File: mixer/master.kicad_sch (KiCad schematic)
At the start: 18 parts, among them J1 EURORACK_CONN_16, J2 AUX_OUT, J3 AUX_IN_R, J4 AUX_IN_L, J5 MAIN_OUT_R, J6 MAIN_OUT_L, U1 TL074

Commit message: making progress on the outline
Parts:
- C1, C2, C3, C4: footprint (none) -> Capacitor_SMD:C_0603_1608Metric
- R1, R2, R3, R4, R5: footprint (none) -> Resistor_SMD:R_0603_1608Metric
- U1: footprint (none) -> Package_SO:SOIC-14_3.9x8.7mm_P1.27mm
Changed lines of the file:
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@@
 			)
 		)
-		(property "Footprint" ""
+		(property "Footprint" "Resistor_SMD:R_0603_1608Metric"
 			(at 83.312 34.29 90)
 			(effects
@@
 			)
 		)
-		(property "Footprint" ""
+		(property "Footprint" "Capacitor_SMD:C_0603_1608Metric"
 			(at 275.2852 35.56 0)
 			(effects
@@
 			)
 		)
-		(property "Footprint" ""
+		(property "Footprint" "Resistor_SMD:R_0603_1608Metric"
 			(at 152.4 128.778 90)
 			(effects
@@
 			)
 		)
-		(property "Footprint" ""
+		(property "Footprint" "Package_SO:SOIC-14_3.9x8.7mm_P1.27mm"
 			(at 170.18 109.22 0)
 			(effects
@@
 			)
 		)
-		(property "Footprint" ""
+		(property "Footprint" "Capacitor_SMD:C_0603_1608Metric"
 			(at 33.9852 43.18 0)
 			(effects
@@
 			)
 		)
-		(property "Footprint" ""
+		(property "Footprint" "Resistor_SMD:R_0603_1608Metric"
 			(at 152.4 141.478 90)
 			(effects
@@
 			)
 		)
-		(property "Footprint" ""
+		(property "Footprint" "Resistor_SMD:R_0603_1608Metric"
 			(at 152.4 93.218 90)
 			(effects
@@
 			)
 		)
-		(property "Footprint" ""
+		(property "Footprint" "Capacitor_SMD:C_0603_1608Metric"
 			(at 20.0152 31.75 0)
 			(effects
@@
 			)
 		)
-		(property "Footprint" ""
+		(property "Footprint" "Package_SO:SOIC-14_3.9x8.7mm_P1.27mm"
 			(at 130.81 88.9 0)
 			(effects
@@
 			)
 		)
-		(property "Footprint" ""
+		(property "Footprint" "Package_SO:SOIC-14_3.9x8.7mm_P1.27mm"
 			(at 170.18 144.78 0)
 			(effects
@@
 			)
 		)
-		(property "Footprint" ""
+		(property "Footprint" "Resistor_SMD:R_0603_1608Metric"
 			(at 152.4 105.918 90)
 			(effects
@@
 			)
 		)
-		(property "Footprint" ""
+		(property "Footprint" "Package_SO:SOIC-14_3.9x8.7mm_P1.27mm"
 			(at 262.89 29.21 0)
 			(effects
@@
 			)
 		)
-		(property "Footprint" ""
+		(property "Footprint" "Package_SO:SOIC-14_3.9x8.7mm_P1.27mm"
 			(at 134.62 137.16 0)
 			(effects
@@
 			)
 		)
-		(property "Footprint" ""
+		(property "Footprint" "Capacitor_SMD:C_0603_1608Metric"
 			(at 33.9852 31.75 0)
 			(effects

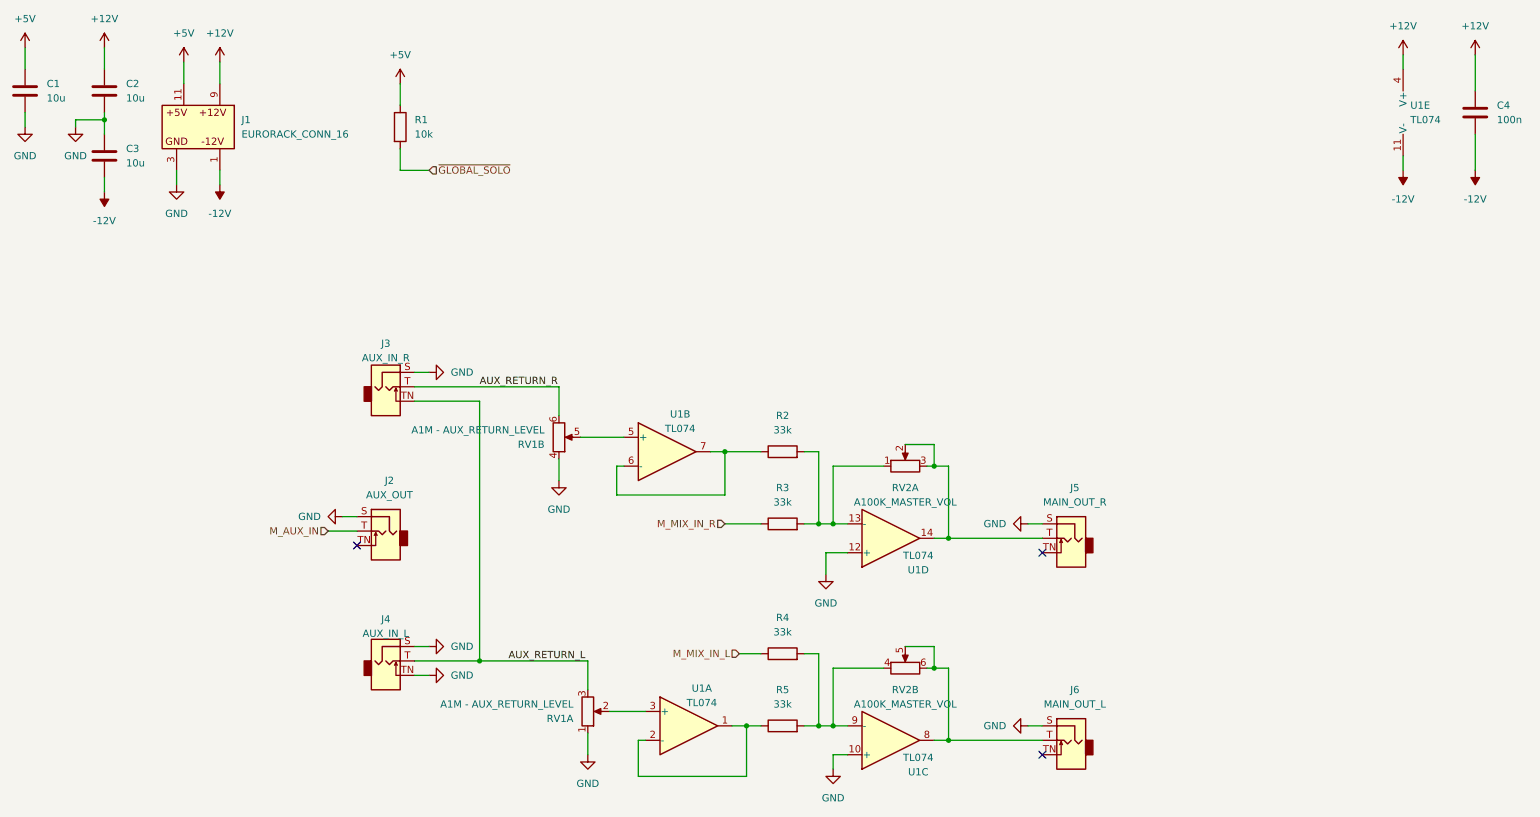
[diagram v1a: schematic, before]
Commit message: layed out parts
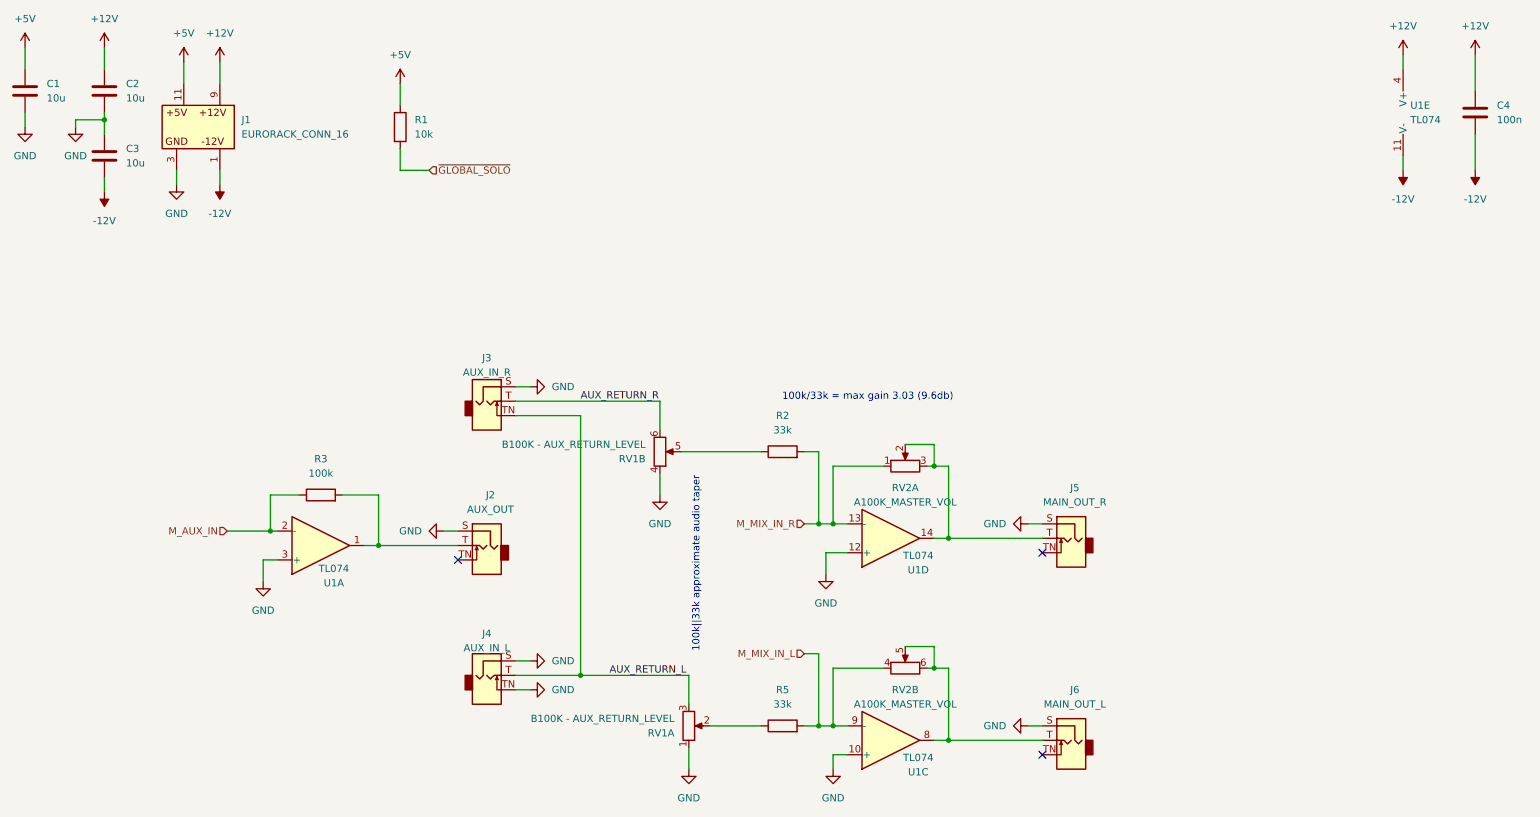
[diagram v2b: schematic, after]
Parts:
- removed R4: 33k, Resistor_SMD:R_0603_1608Metric, symbol Device:R
- removed unit 2 of U1
- R3: value 33k -> 100k
- RV1: value A1M - AUX_RETURN_LEVEL -> B100K - AUX_RETURN_LEVEL
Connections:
- net GND: now also U1.3 (+)
- net M_AUX_IN: now also R3.1, U1.2 (-); no longer J2.T
- net M_MIX_IN_L: now also R5.2, RV2.4, U1.9 (-)
- net M_MIX_IN_R: now also R2.2, RV2.1, U1.13 (-); no longer R3.1
- net at RV1.2: now also R5.1; no longer U1.3 (+)
- net at R2.1: now also RV1.5
- new net: J2.T, R3.2, U1.1
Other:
- note added: "100k/33k = max gain 3.03 (9.6db)"
- note added: "100k||33k approximate audio taper"
- moved on the sheet: J2, J3, J4, RV1A, RV1B
